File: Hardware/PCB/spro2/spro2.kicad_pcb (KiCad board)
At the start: 2 copper layers, 102.2 x 64 mm, 44 parts, among them J2 MAX30102, J3 Humidity sensor, U1 LM35-LP, U2 OPA340P, U3 TL074

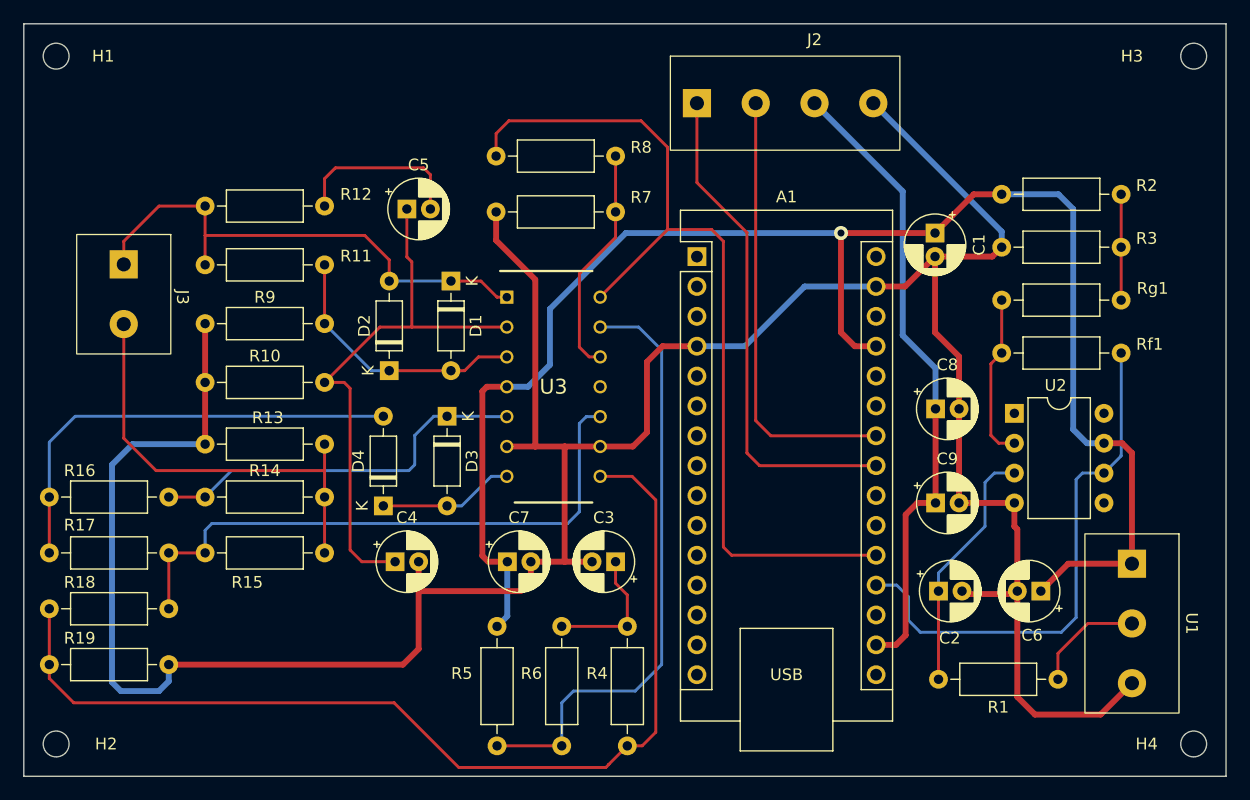
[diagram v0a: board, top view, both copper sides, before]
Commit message: Second version of the PCB
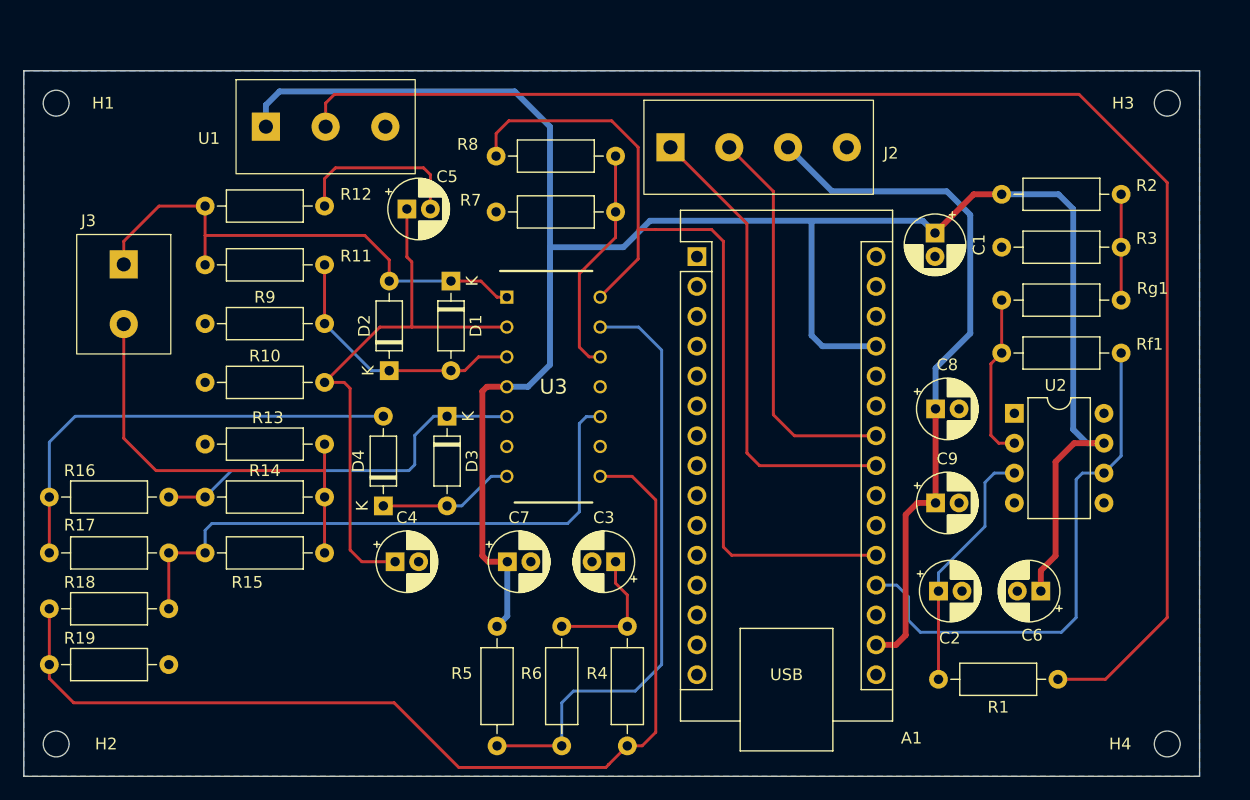
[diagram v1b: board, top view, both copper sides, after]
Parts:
- moved U1 80.5 mm to (100.7, 84.0), turned to 0 degrees
- moved H3 4.59 mm to (172.2, 82.0)
- moved J2 4.37 mm to (140.0, 85.8)
- moved H1 4.00 mm to (77.8, 82.0)
- moved H4 2.25 mm to (172.2, 136.5)
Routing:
- net GND: track 250.1 -> 0.00 mm
- net /Temperature sensor filter and amplifier/Temp_In: track 9.55 -> 125.5 mm
- net +5V: track 137.3 -> 183.4 mm, vias 1 -> 0
- net +3.3V: track 54.3 -> 59.7 mm
- net Net-(A1-A5): track 37.8 -> 33.8 mm
- net Net-(A1-A4): track 42.9 -> 40.1 mm
- net /Humidity: track 77.4 -> 76.4 mm
- added copper zone on B.Cu, net GND
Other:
- board size 102.2 x 64 mm -> 100 x 60 mm
